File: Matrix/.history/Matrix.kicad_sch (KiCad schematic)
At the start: 13 parts

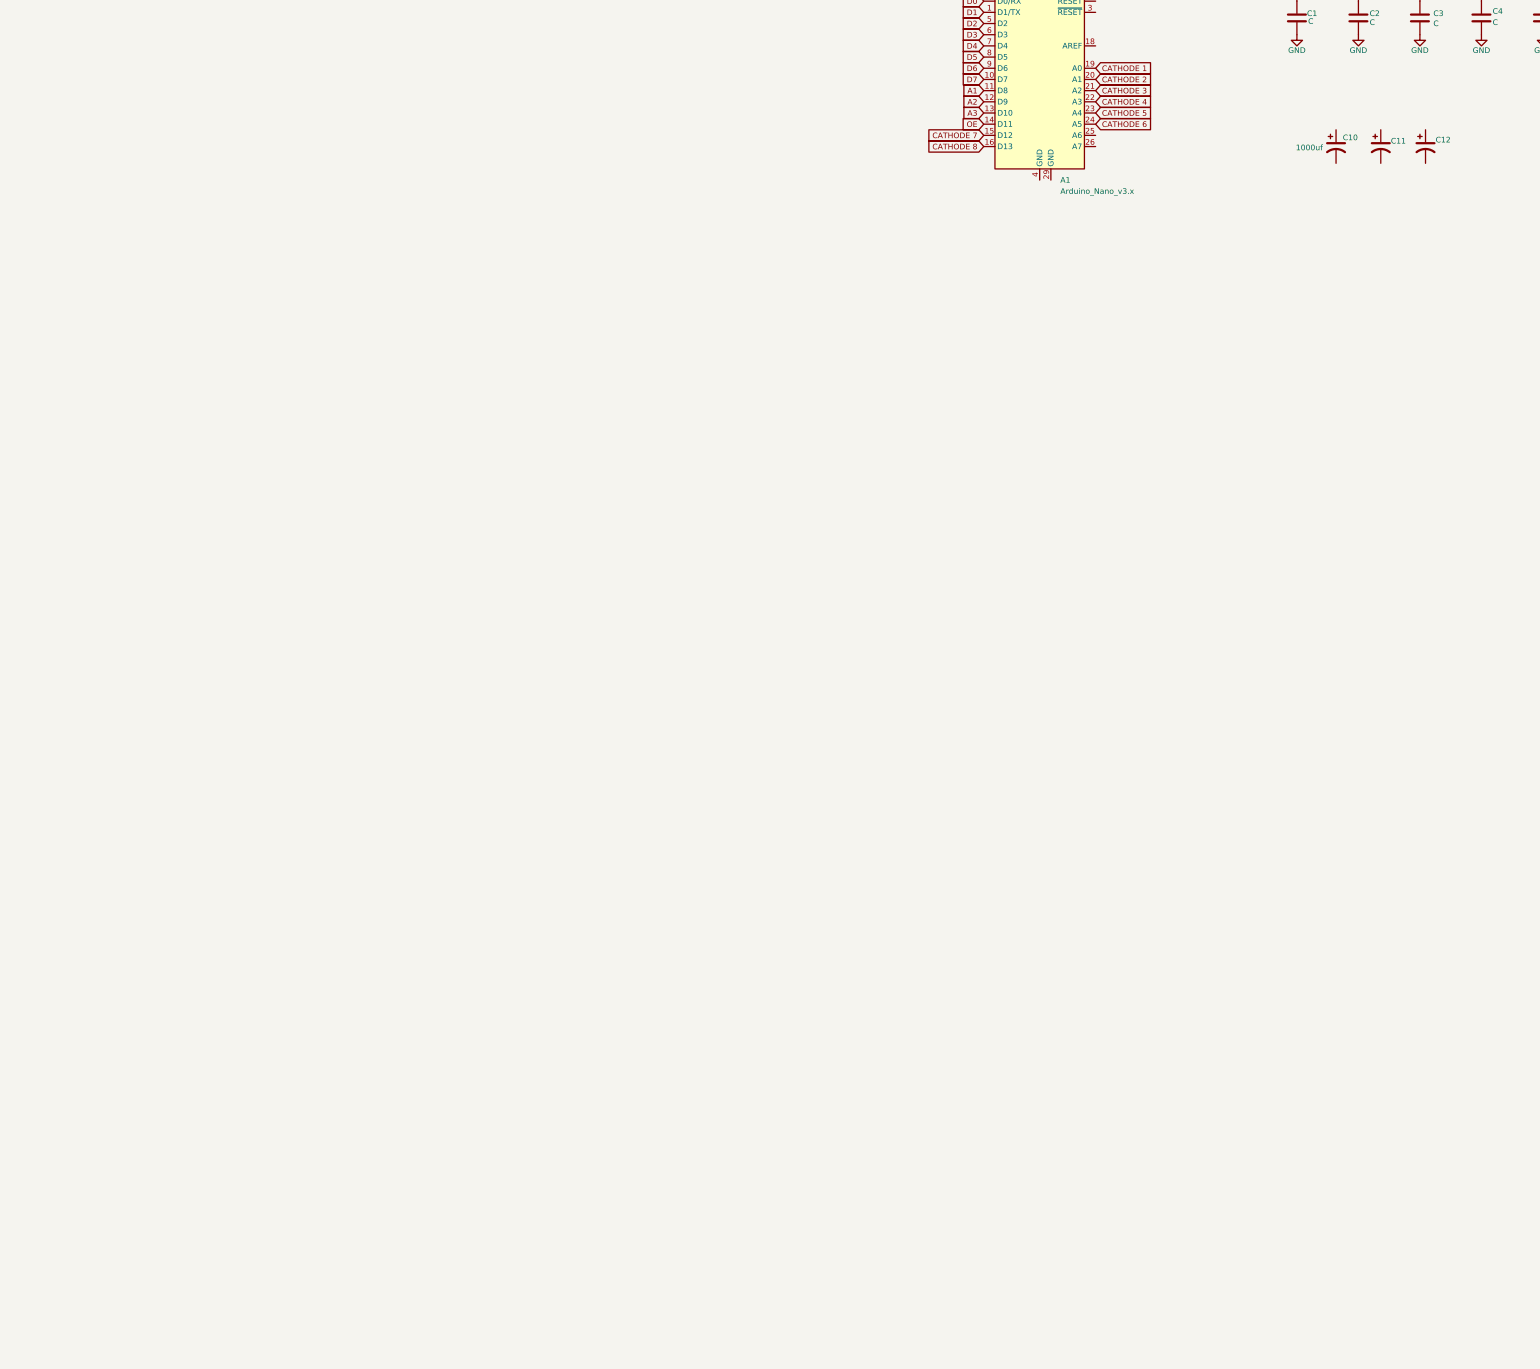
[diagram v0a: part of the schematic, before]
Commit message: Update Matrix.kicad_sch
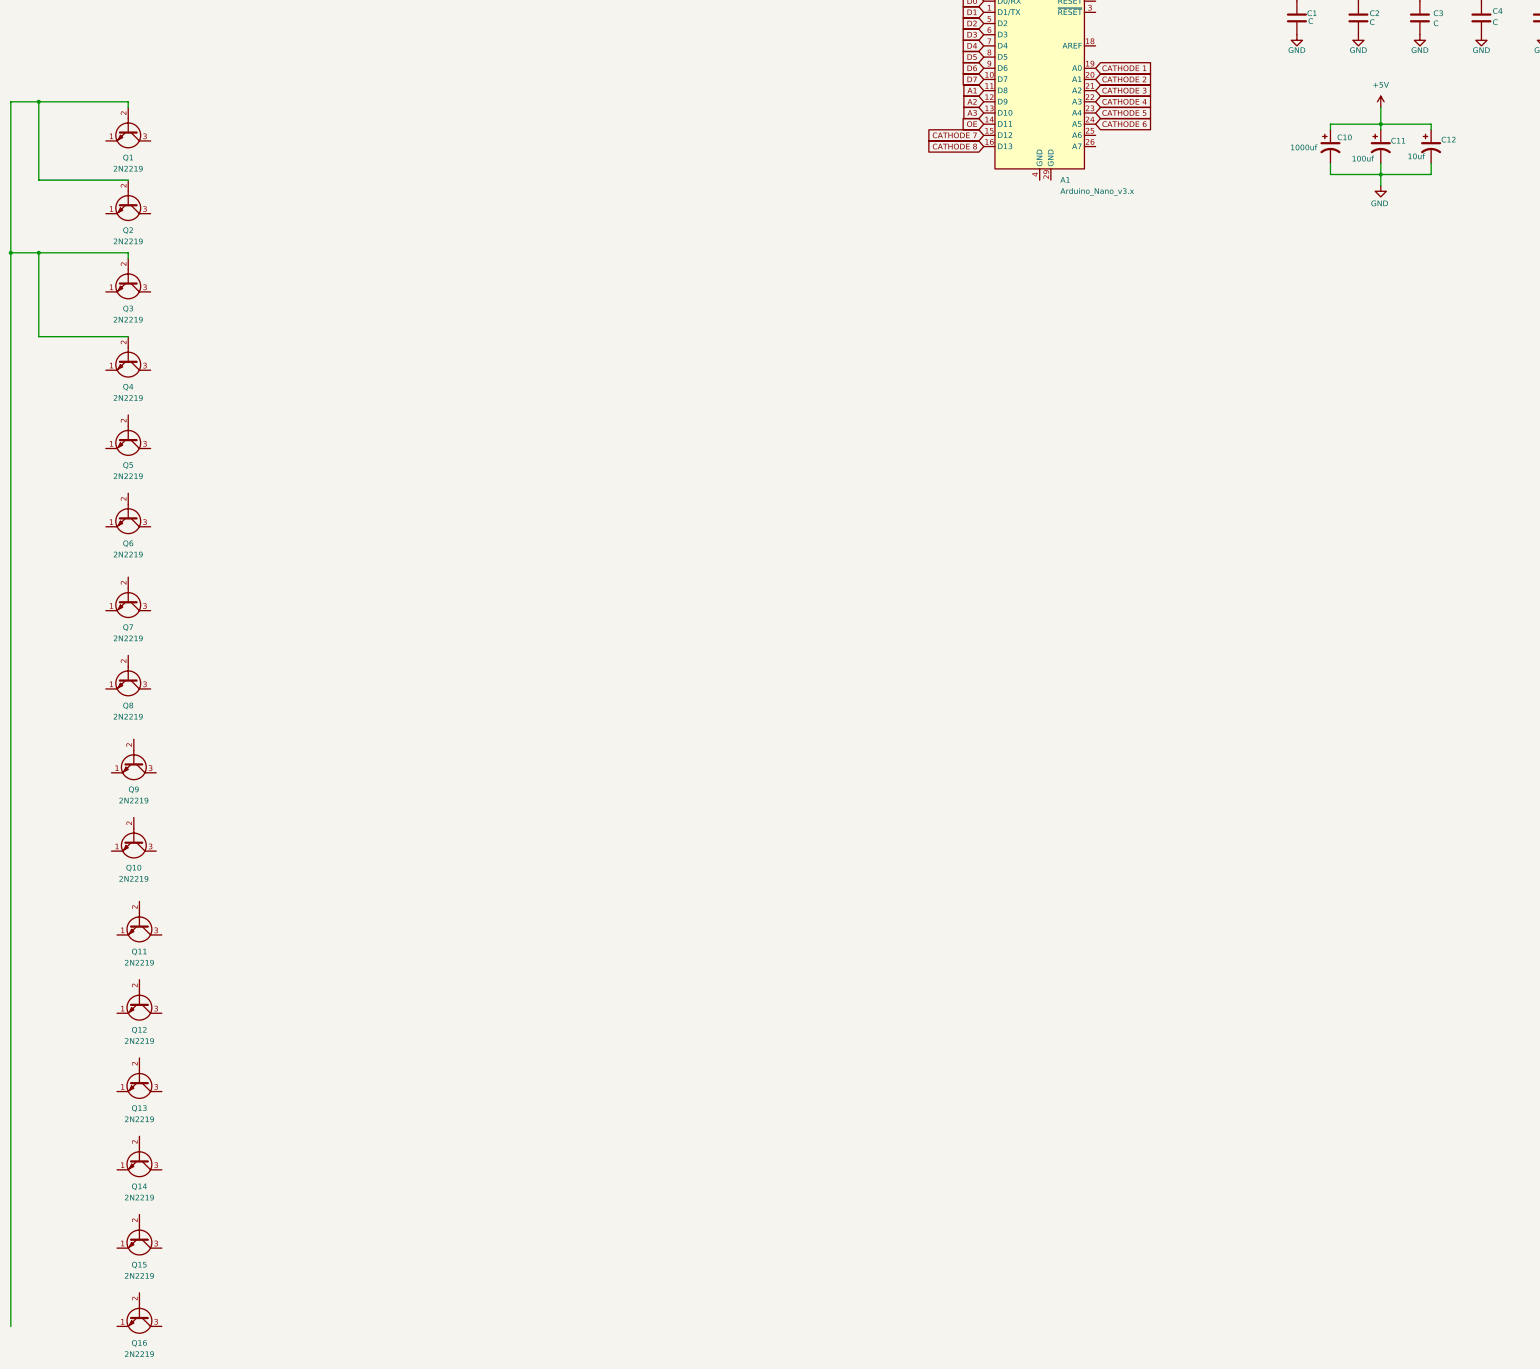
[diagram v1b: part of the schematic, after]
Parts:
- added Q1, Q10, Q11, Q12, Q13, Q14, Q15, Q16, Q2, Q3, Q4, Q5, Q6, Q7, Q8, Q9: 2N2219, Package_TO_SOT_THT:TO-39-3, symbol Transistor_BJT:2N2219
- C11: value C_Polarized_US -> 100uf
- C12: value C_Polarized_US -> 10uf
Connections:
- net +5V: now also C10.1, C11.1, C12.1
- net GND: now also C10.2, C11.2, C12.2
- new net: Q1.2 (B), Q2.2 (B), Q3.2 (B), Q4.2 (B)
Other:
- moved on the sheet: C10, C12

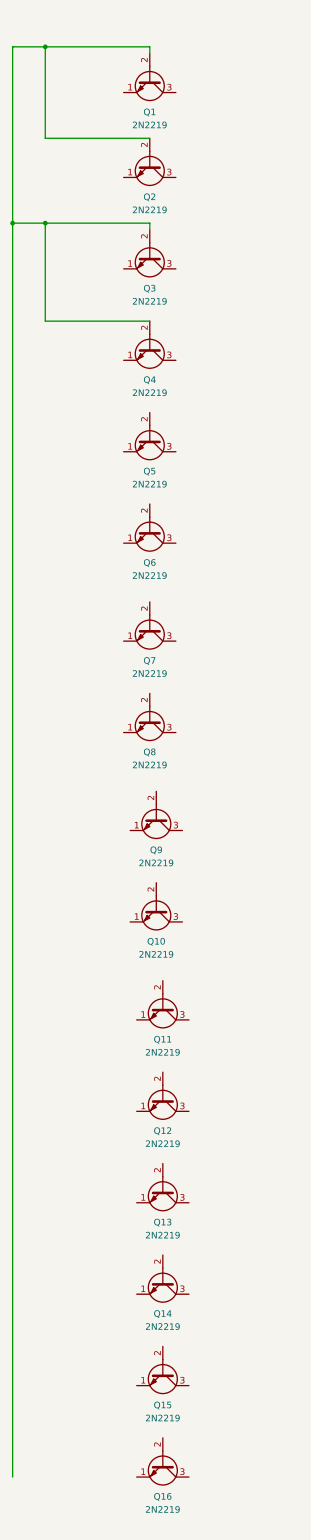
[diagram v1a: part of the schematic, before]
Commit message: Update Matrix.kicad_sch
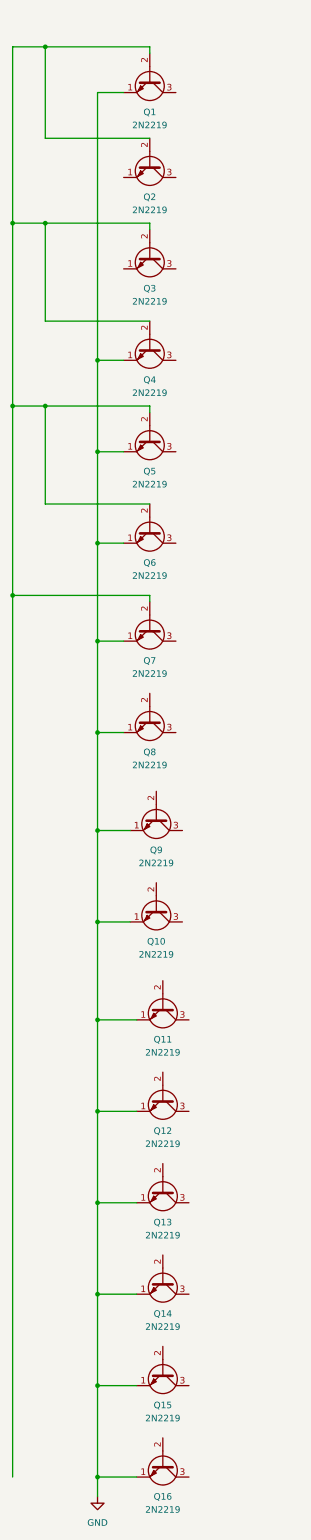
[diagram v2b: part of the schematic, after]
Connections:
- net GND: now also Q1.1 (E), Q10.1 (E), Q11.1 (E), Q12.1 (E), Q13.1 (E), Q14.1 (E), Q15.1 (E), Q16.1 (E), Q4.1 (E), Q5.1 (E), Q6.1 (E), Q7.1 (E), Q8.1 (E), Q9.1 (E)
- net at Q1.2 (B), Q2.2 (B), Q3.2 (B)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: now also Q5.2 (B), Q6.2 (B), Q7.2 (B)

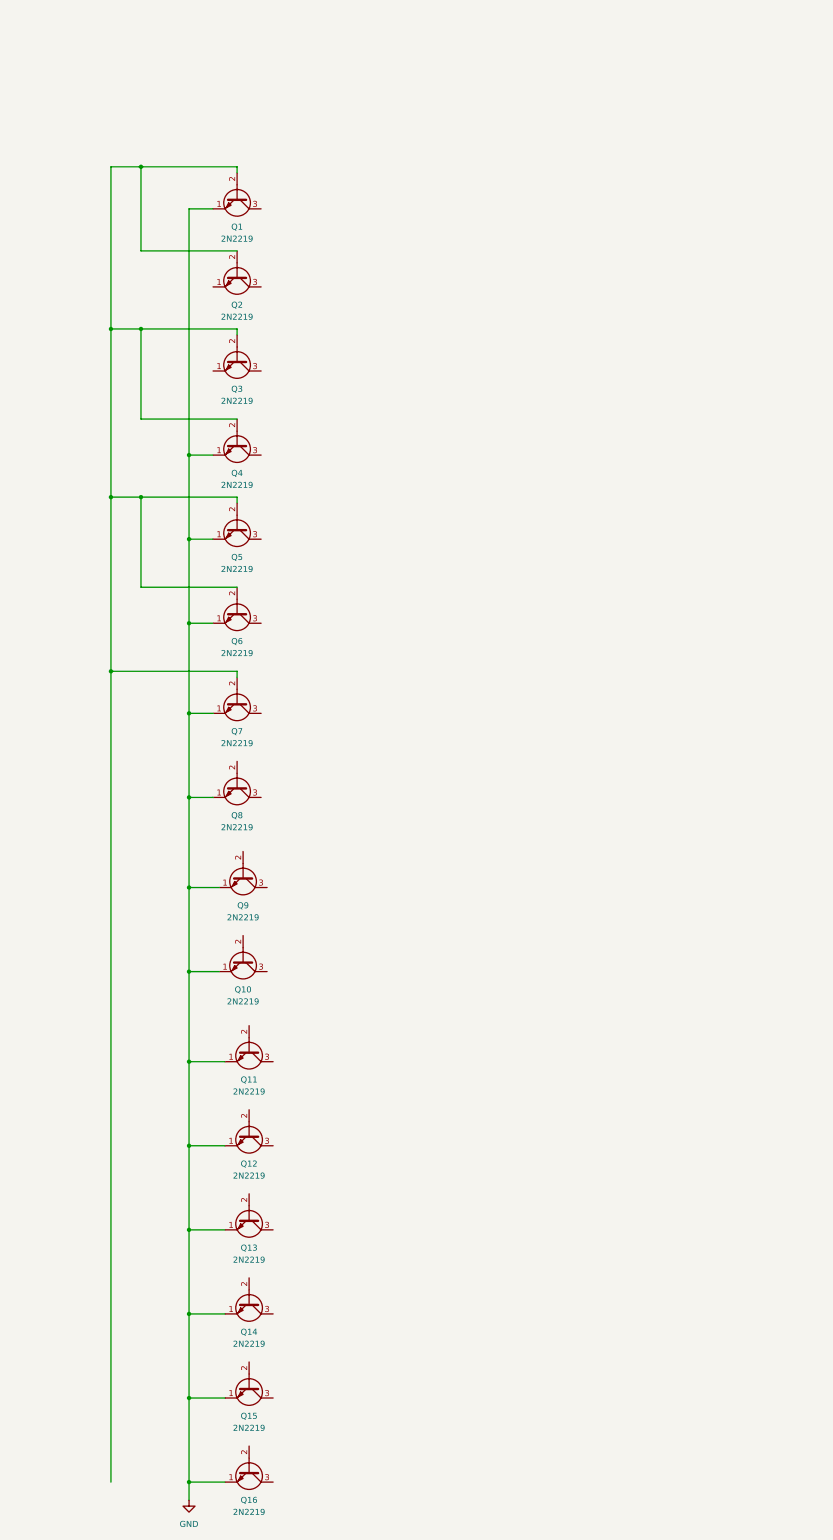
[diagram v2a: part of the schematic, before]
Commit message: Update Matrix.kicad_sch
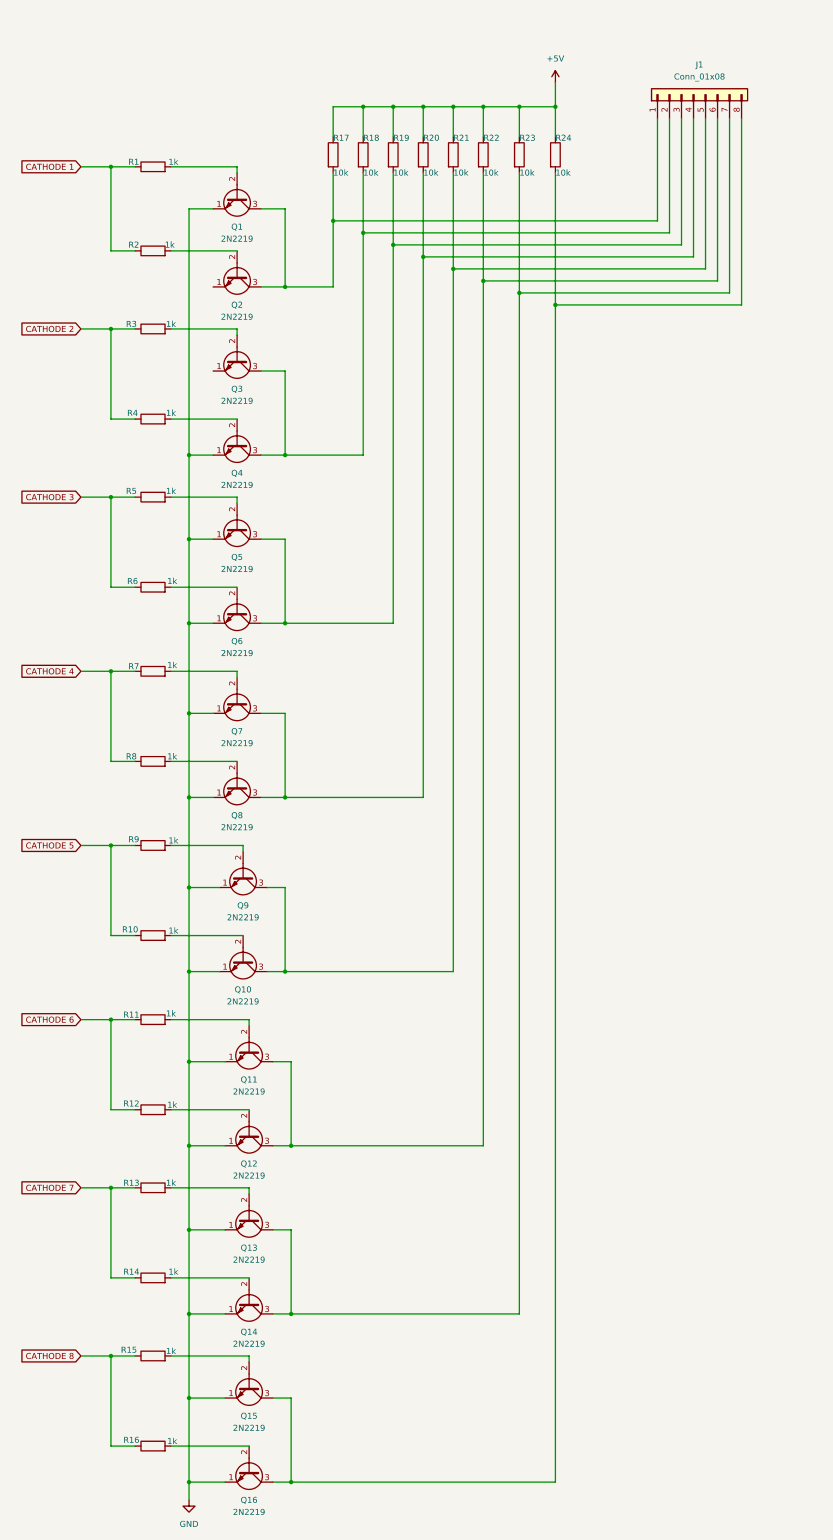
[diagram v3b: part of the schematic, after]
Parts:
- added J1: Conn_01x08, symbol Connector_Generic:Conn_01x08
- added R1, R10, R11, R12, R13, R14, R15, R16, R2, R3, R4, R5, R6, R7, R8, R9: 1k, symbol Device:R
- added R17, R18, R19, R20, R21, R22, R23, R24: 10k, symbol Device:R
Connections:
- net +5V: now also R17.1, R18.1, R19.1, R20.1, R21.1, R22.1, R23.1, R24.1
- net CATHODE 1: now also R1.1, R2.1
- net CATHODE 2: now also R3.1, R4.1
- net CATHODE 3: now also R5.1, R6.1
- net CATHODE 4: now also R7.1, R8.1
- net CATHODE 5: now also R10.1, R9.1
- net CATHODE 6: now also R11.1, R12.1
- net CATHODE 7: now also R13.1, R14.1
- net CATHODE 8: now also R15.1, R16.1
- net at Q1.3 (C): now also Q2.3 (C), J1.1 (Pin_1), R17.2
- net at Q13.2 (B): now also R13.2
- net at Q13.3 (C): now also Q14.3 (C), J1.7 (Pin_7), R23.2
- net at Q16.2 (B): now also R16.2
- net at Q16.3 (C): now also Q15.3 (C), J1.8 (Pin_8), R24.2
- net at Q11.2 (B): now also R11.2
- net at Q11.3 (C): now also Q12.3 (C), J1.6 (Pin_6), R22.2
- net at Q15.2 (B): now also R15.2
- net at Q7.3 (C): now also Q8.3 (C), J1.4 (Pin_4), R20.2
- net at Q5.3 (C): now also Q6.3 (C), J1.3 (Pin_3), R19.2
- net at Q8.2 (B): now also R8.2
- net at Q12.2 (B): now also R12.2
- net at Q14.2 (B): now also R14.2
- net at Q9.2 (B): now also R9.2
- net at Q9.3 (C): now also Q10.3 (C), J1.5 (Pin_5), R21.2
- net at Q10.2 (B): now also R10.2
- net at Q3.3 (C): now also Q4.3 (C), J1.2 (Pin_2), R18.2
- new net: Q5.2 (B), R5.2
- new net: Q1.2 (B), R1.2
- new net: Q3.2 (B), R3.2
- new net: Q7.2 (B), R7.2
- new net: Q2.2 (B), R2.2
- new net: Q6.2 (B), R6.2
- new net: Q4.2 (B), R4.2

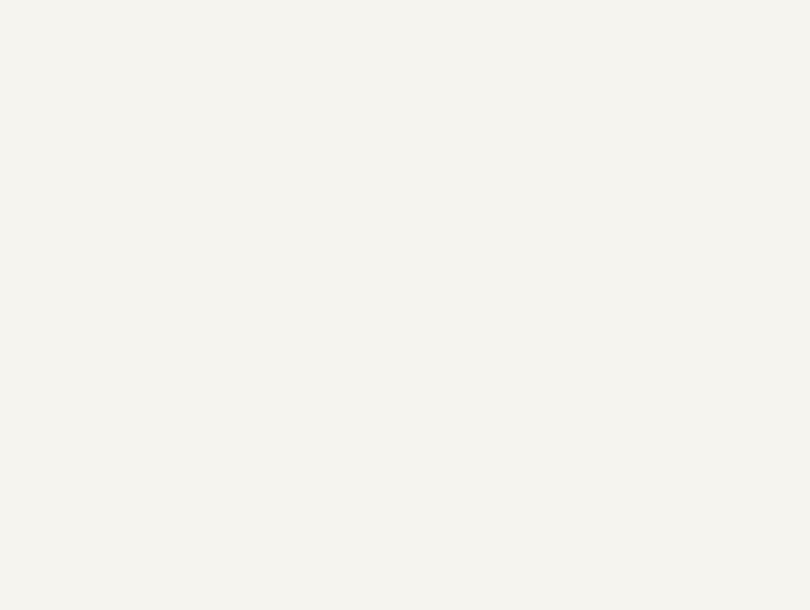
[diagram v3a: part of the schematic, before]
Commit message: Update Matrix.kicad_sch
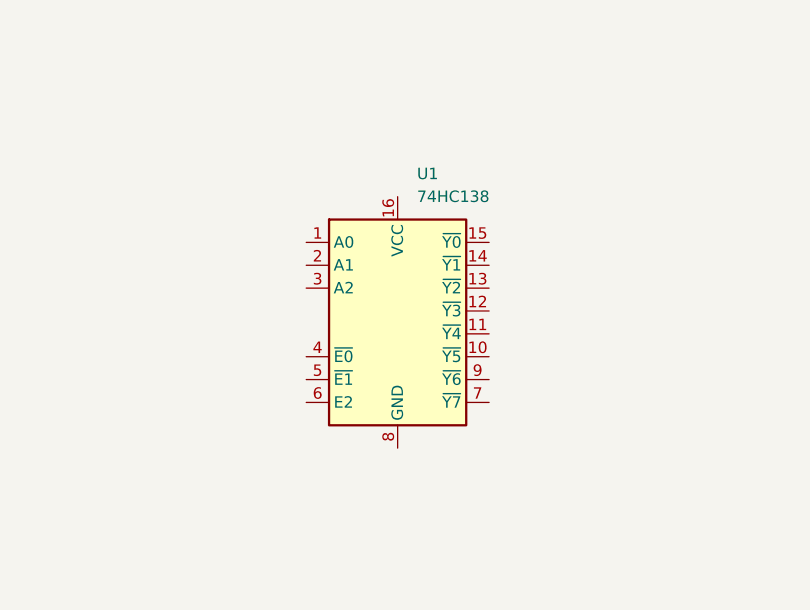
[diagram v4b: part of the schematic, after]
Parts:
- added U1: 74HC138, symbol 74xx:74HC138
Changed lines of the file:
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@@
+	)
+	(symbol
+		(lib_id "74xx:74HC138")
+		(at 237.49 251.46 0)
+		(unit 1)
+		(body_style 1)
+		(exclude_from_sim no)
+		(in_bom yes)
+		(on_board yes)
+		(in_pos_files yes)
+		(dnp no)
+		(fields_autoplaced yes)
+		(property "Reference" "U1"
+			(at 239.6333 233.68 0)
+			(show_name no)
+			(do_not_autoplace no)
+			(effects
+				(font
+					(size 1.27 1.27)
+				)
+				(justify left)
+			)
+		)
+		(property "Value" "74HC138"
+			(at 239.6333 236.22 0)
+			(show_name no)
+			(do_not_autoplace no)
+			(effects
+				(font
+					(size 1.27 1.27)
+				)
+				(justify left)
+			)
+		)
+		(property "Footprint" ""
+			(at 237.49 251.46 0)
+			(hide yes)
+			(show_name no)
+			(do_not_autoplace no)
+			(effects
+				(font
+					(size 1.27 1.27)
+				)
+			)
+		)
+		(property "Datasheet" "http://www.ti.com/lit/ds/symlink/cd74hc238.pdf"
+			(at 237.49 251.46 0)
+			(hide yes)
+			(show_name no)
+			(do_not_autoplace no)
+			(effects
+				(font
+					(size 1.27 1.27)
+				)
+			)
+		)
+		(property "Description" "3-to-8 line decoder/multiplexer inverting, DIP-16/SOIC-16/SSOP-16"
+			(at 237.49 251.46 0)
+			(hide yes)
+			(show_name no)
+			(do_not_autoplace no)
+			(effects
+				(font
+					(size 1.27 1.27)
+				)
+			)
+		)
+		(pin "5"
+		)
+		(pin "13"
+		)
+		(pin "11"
+		)
+		(pin "10"
+		)
+		(pin "6"
+		)
+		(pin "9"
+		)
+		(pin "8"
+		)
+		(pin "4"
+		)
+		(pin "12"
+		)
+		(pin "7"
+		)
+		(pin "3"
+		)
+		(pin "16"
+		)
+		(pin "14"
+		)
+		(pin "1"
+		)
+		(pin "2"
+		)
+		(pin "15"
+		)
+		(instances
+			(project "Matrix"
+				(path "/88b088a6-0f2a-4bb0-891c-efec1204d77b"
+					(reference "U1")
+					(unit 1)
+				)
+			)
+		)
 	)
 	(symbol
